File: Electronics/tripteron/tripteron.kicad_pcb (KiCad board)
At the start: 2 copper layers, 100 x 100 mm, 27 parts, among them J1 Conn_01x02_Pin, J2 Conn_01x04_Pin, J3 Conn_01x04_Pin, J4 Conn_01x04_Pin, J5 Conn_01x04_Pin, J6 Conn_01x04_Pin

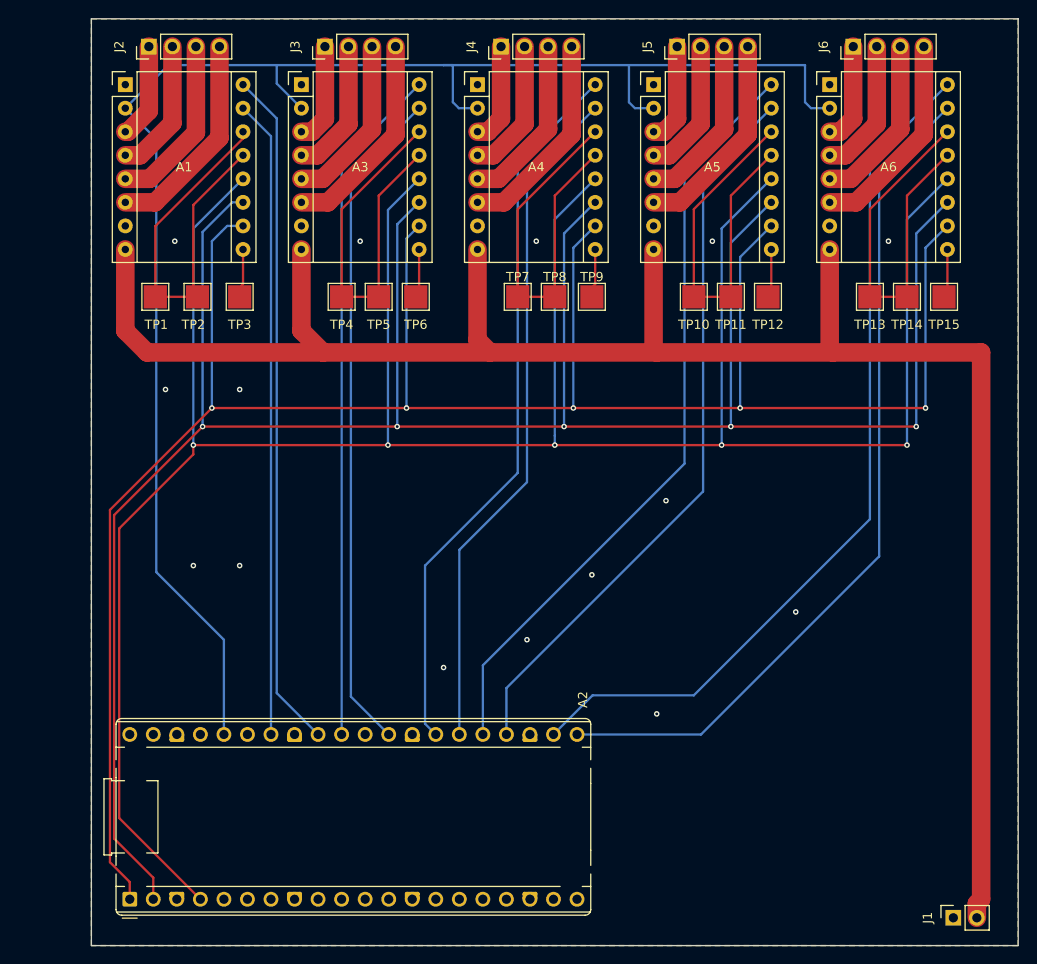
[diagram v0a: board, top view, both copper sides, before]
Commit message: uncertanty and V2 boards
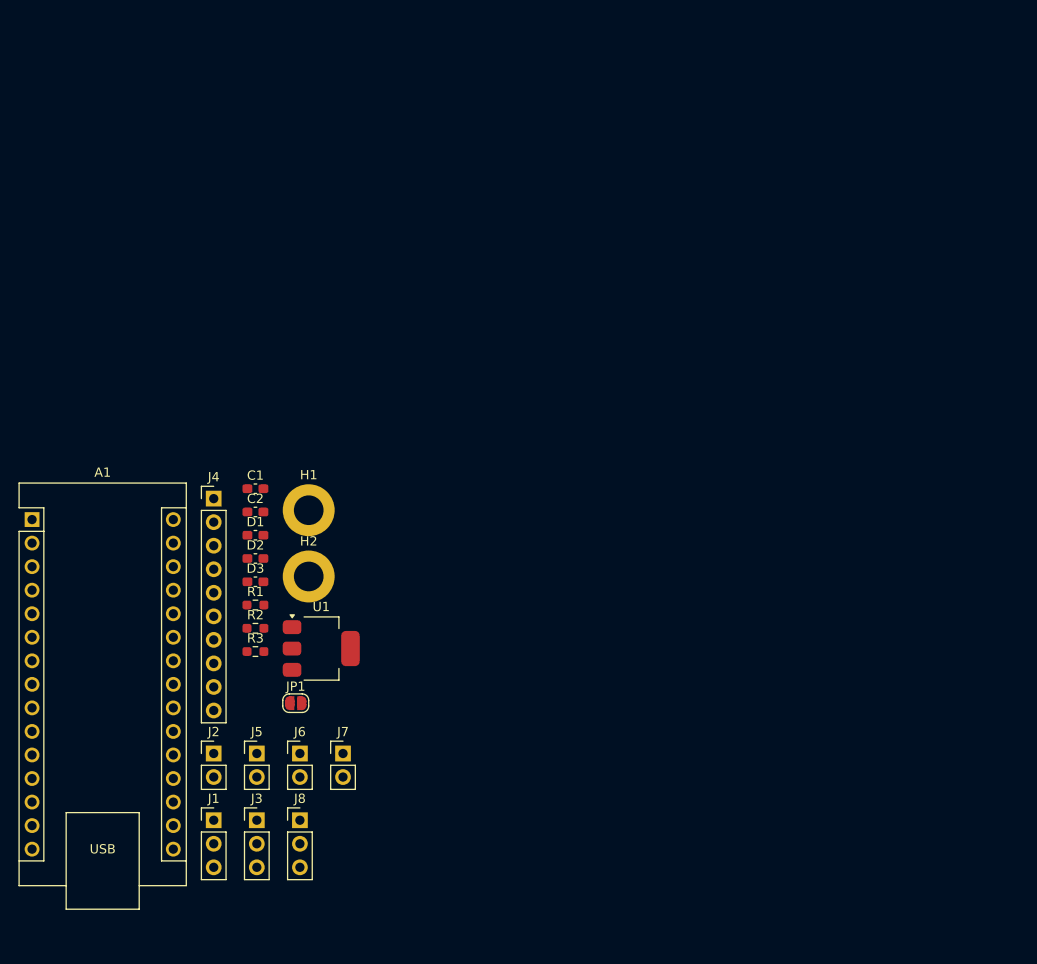
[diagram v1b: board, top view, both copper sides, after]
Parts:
- removed A2: RaspberryPi_Pico, Module:RaspberryPi_Pico_Common_THT
- removed A3, A4, A5, A6: Pololu_Breakout_A4988, Module:Pololu_Breakout-16_15.2x20.3mm
- removed TP1, TP10, TP11, TP12, TP13, TP14, TP15, TP2, TP3, TP4, TP5, TP6, TP7, TP8, TP9: TestPoint, TestPoint:TestPoint_Pad_2.5x2.5mm
- added C1: C, Capacitor_SMD:C_0603_1608Metric_Pad1.08x0.95mm_HandSolder, F.Cu at (97.7, 90.7)
- added C2: C, Capacitor_SMD:C_0603_1608Metric_Pad1.08x0.95mm_HandSolder, F.Cu at (97.7, 93.2)
- added D1: LED, Capacitor_SMD:C_0603_1608Metric_Pad1.08x0.95mm_HandSolder, F.Cu at (97.7, 95.7)
- added D2: LED, Capacitor_SMD:C_0603_1608Metric_Pad1.08x0.95mm_HandSolder, F.Cu at (97.7, 98.2)
- added D3: LED, Capacitor_SMD:C_0603_1608Metric_Pad1.08x0.95mm_HandSolder, F.Cu at (97.7, 100.7)
- added H1: MountingHole_Pad, MountingHole:MountingHole_3.2mm_M3_DIN965_Pad, F.Cu at (103.5, 93.0)
- added H2: MountingHole_Pad, MountingHole:MountingHole_3.2mm_M3_DIN965_Pad, F.Cu at (103.5, 100.2)
- added J7: Conn_01x02_Pin, Connector_PinHeader_2.54mm:PinHeader_1x02_P2.54mm_Vertical, F.Cu at (107.2, 119.3)
- added J8: Conn_01x03_Pin, Connector_PinHeader_2.54mm:PinHeader_1x03_P2.54mm_Vertical, F.Cu at (102.5, 126.5)
- added JP1: SolderJumper_2_Open, Jumper:SolderJumper-2_P1.3mm_Open_RoundedPad1.0x1.5mm, F.Cu at (102.0, 113.8)
- added R1: R, Resistor_SMD:R_0603_1608Metric_Pad0.98x0.95mm_HandSolder, F.Cu at (97.7, 103.3)
- added R2: R, Resistor_SMD:R_0603_1608Metric_Pad0.98x0.95mm_HandSolder, F.Cu at (97.7, 105.8)
- added R3: R, Resistor_SMD:R_0603_1608Metric_Pad0.98x0.95mm_HandSolder, F.Cu at (97.7, 108.3)
- added U1: NCP1117-3.3_SOT223, Package_TO_SOT_SMD:SOT-223-3_TabPin2, F.Cu at (104.8, 108.0)
- A1: value Pololu_Breakout_A4988 -> Arduino_Nano_RP2040_Connect; footprint Module:Pololu_Breakout-16_15.2x20.3mm -> Module:Arduino_Nano
- J1: value Conn_01x02_Pin -> Conn_01x03_Pin; footprint Connector_PinSocket_2.54mm:PinSocket_1x02_P2.54mm_Vertical -> Connector_PinHeader_2.54mm:PinHeader_1x03_P2.54mm_Vertical
- J2, J5, J6: value Conn_01x04_Pin -> Conn_01x02_Pin; footprint Connector_PinHeader_2.54mm:PinHeader_1x04_P2.54mm_Vertical -> Connector_PinHeader_2.54mm:PinHeader_1x02_P2.54mm_Vertical
- J3: value Conn_01x04_Pin -> Conn_01x03_Pin; footprint Connector_PinHeader_2.54mm:PinHeader_1x04_P2.54mm_Vertical -> Connector_PinHeader_2.54mm:PinHeader_1x03_P2.54mm_Vertical
- J4: value Conn_01x04_Pin -> Conn_01x10_Pin; footprint Connector_PinHeader_2.54mm:PinHeader_1x04_P2.54mm_Vertical -> Connector_PinHeader_2.54mm:PinHeader_1x10_P2.54mm_Vertical
- moved J6 96.9 mm to (102.5, 119.3), turned to 0 degrees
- moved J5 88.7 mm to (97.8, 119.3), turned to 0 degrees
- moved J3 83.8 mm to (97.8, 126.5), turned to 0 degrees
- moved J1 80.5 mm to (93.2, 126.5), turned to 0 degrees
- moved J2 76.6 mm to (93.2, 119.3), turned to 0 degrees
- moved J4 57.8 mm to (93.2, 91.8), turned to 0 degrees
- moved A1 48.0 mm to (73.6, 94.0)
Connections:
- A1 pad 1: GND -> unconnected-(A1-D1/TX-Pad1)
- A1 pad 10: MS1 -> M3_STP
- A1 pad 11: MS2 -> XSHUT_1
- A1 pad 12: MS3 -> XSHUT_2
- A1 pad 13: /RST_M1 -> XSHUT_3
- A1 pad 14: /RST_M1 -> INT_1
- A1 pad 15: STP_M1 -> INT_2
- A1 pad 16: DIR_M1 -> INT_3
- A1 pad 2: +3.3V -> unconnected-(A1-D0/RX-Pad2)
- A1 pad 3: 1B_M1 -> unconnected-(A1-~{RESET}-Pad3)
- A1 pad 4: 1A_M1 -> GND
- A1 pad 5: 2A_M1 -> M1_DIR
- A1 pad 6: 2B_M1 -> M1_STP
- A1 pad 7: GND -> M2_DIR
- A1 pad 8: +12V -> M2_STP
- A1 pad 9: /EN_M1 -> M3_DIR
- J1 pad 1: GND -> XSHUT_3
- J1 pad 2: +12V -> XSHUT_2
- J2 pad 1: 1B_M1 -> M1_STP
- J2 pad 2: 1A_M1 -> M1_DIR
- J3 pad 1: 1B_M2 -> INT_3
- J3 pad 2: 1A_M2 -> INT_2
- J3 pad 3: 2A_M2 -> INT_1
- J4 pad 1: 1B_M3 -> GND
- J4 pad 2: 1A_M3 -> GND
- J4 pad 3: 2A_M3 -> GND
- J4 pad 4: 2B_M3 -> GND
- J5 pad 1: 1B_M4 -> M2_STP
- J5 pad 2: 1A_M4 -> M2_DIR
- J6 pad 1: 1B_M5 -> SCL
- J6 pad 2: 1A_M5 -> SDA
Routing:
- net MS3: track 286.0 -> 0.00 mm, vias 5 -> 0
- net MS2: track 262.7 -> 0.00 mm, vias 5 -> 0
- net MS1: track 240.0 -> 0.00 mm, vias 5 -> 0
- net +12V: track 209.5 -> 0.00 mm
- net +3.3V: track 174.8 -> 0.00 mm
- net DIR_M5: track 94.1 -> 0.00 mm
- net STP_M5: track 92.0 -> 0.00 mm
- net DIR_M4: track 83.0 -> 0.00 mm
- net STP_M4: track 79.4 -> 0.00 mm
- net DIR_M3: track 78.2 -> 0.00 mm
- net STP_M3: track 73.6 -> 0.00 mm
- net DIR_M2: track 73.6 -> 0.00 mm
- net DIR_M1: track 73.5 -> 0.00 mm
- net STP_M2: track 72.3 -> 0.00 mm
- net STP_M1: track 68.8 -> 0.00 mm
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- removed copper zone on B.Cu, net GND
- removed copper zone on F.Cu, net GND
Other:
- board outline removed
